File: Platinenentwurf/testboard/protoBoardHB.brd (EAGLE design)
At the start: 50 x 46.9 mm, 35 parts, among them U2 STM32F4X5RG

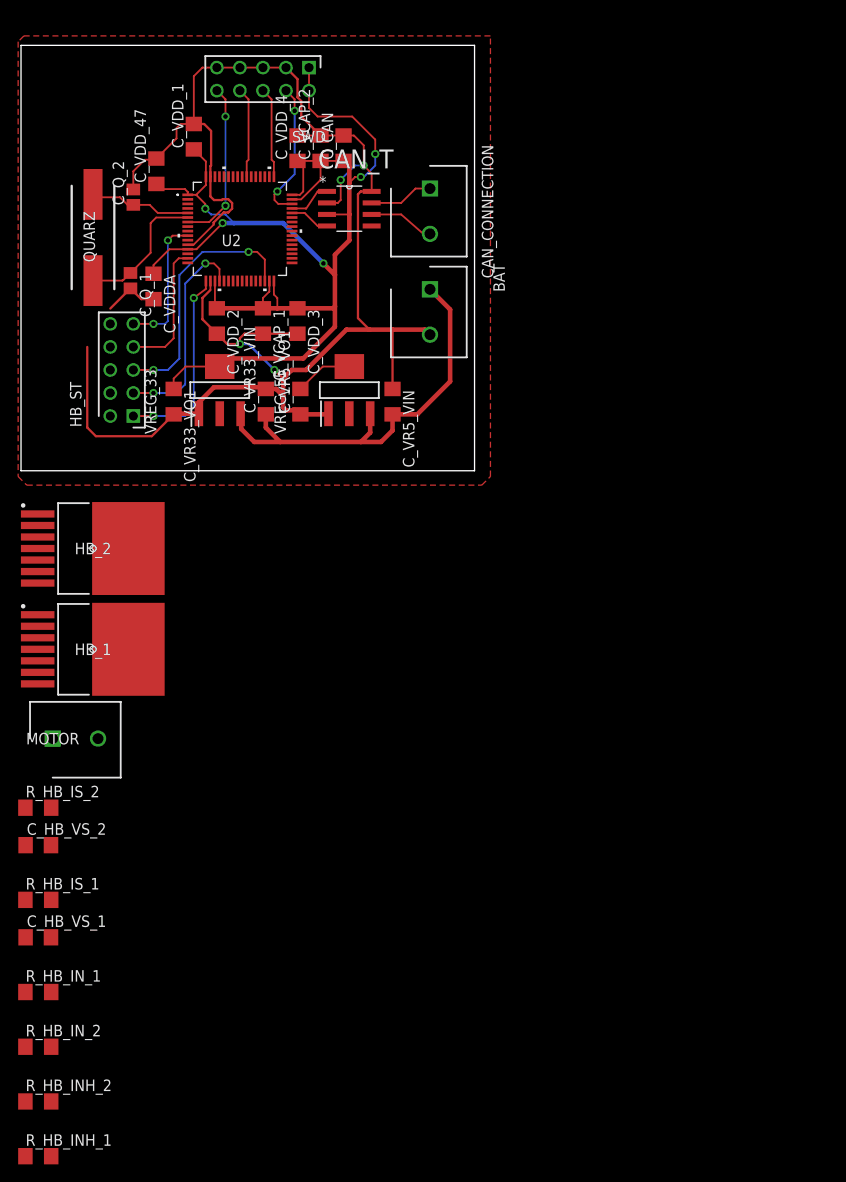
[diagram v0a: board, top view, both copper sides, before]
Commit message: ProtoBoard update
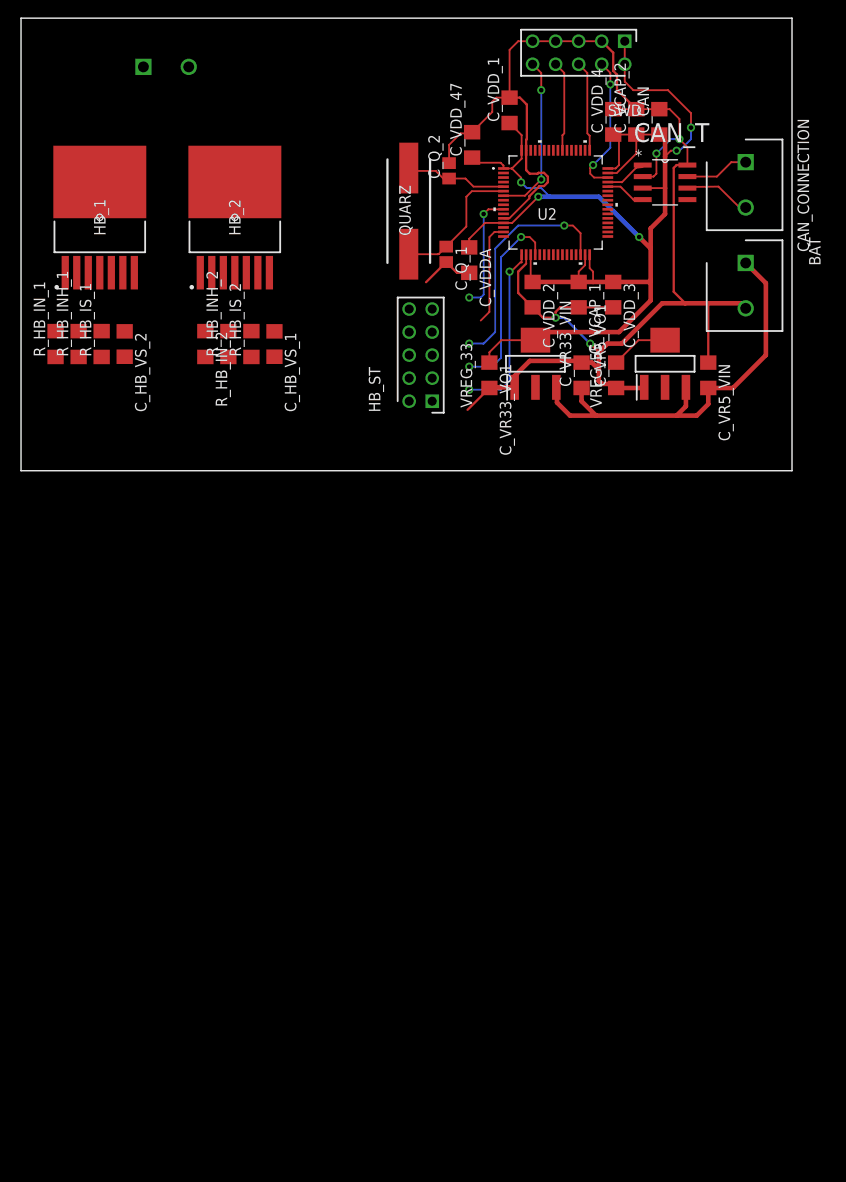
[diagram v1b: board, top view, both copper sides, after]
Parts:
- R_HB_IS_1, R_HB_IS_2: value (none) -> 1k
- moved R_HB_INH_1 89.6 mm to (6.35, 14.0), turned to 90 degrees
- moved R_HB_INH_2 86.1 mm to (22.9, 14.0), turned to 90 degrees
- moved R_HB_IN_2 79.6 mm to (20.3, 14.0), turned to 270 degrees
- moved MOTOR 74.7 mm to (13.5, 44.5), flipped to the bottom, turned to 180 degrees
- moved R_HB_IN_1 71.5 mm to (3.81, 14.0), turned to 90 degrees
- moved C_HB_VS_1 70.4 mm to (27.9, 14.0), turned to 270 degrees
- moved R_HB_IS_1 61.7 mm to (8.89, 14.0), turned to 90 degrees
- moved R_HB_IS_2 56.3 mm to (25.4, 14.0), turned to 90 degrees
- moved C_HB_VS_2 56.1 mm to (11.4, 14.0), turned to 270 degrees
- moved HB_1 47.6 mm to (8.69, 27.9), turned to 90 degrees
- moved HB_2 39.7 mm to (23.6, 27.9), turned to 90 degrees
- moved C_CAN 34.9 mm to (70.4, 38.5)
- moved C_Q_1 34.9 mm to (46.9, 23.9)
- moved C_Q_2 34.9 mm to (47.2, 33.1)
- moved C_VDDA 34.9 mm to (49.4, 23.2)
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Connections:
- removed net N$1: HB_1.4, MOTOR.1
- removed net N$2: HB_2.4, MOTOR.2
- new net V_MOT_MIN: HB_2.8, MOTOR.2
- new net V_MOT_PL: HB_1.8, MOTOR.1
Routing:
- net GND: track 190.8 -> 174.4 mm
- net IN_2: track 14.9 -> 11.4 mm
- net INH: track 15.2 -> 13.0 mm
- net IS_2: track 23.5 -> 21.3 mm
- net IN_1: track 28.0 -> 25.8 mm
- net IS_1: track 21.7 -> 19.5 mm
- removed copper zone on layer 1, net GND
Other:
- board size 50 x 46.9 mm -> 85 x 49.9 mm
